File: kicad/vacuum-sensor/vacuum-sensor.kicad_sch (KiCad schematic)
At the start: 13 parts, among them J1 Conn_01x04, U1 XGZP6857A100KPGPN, U2 XGZP6857A100KPGPN, U3 MIC5233-5.0YM5-TR

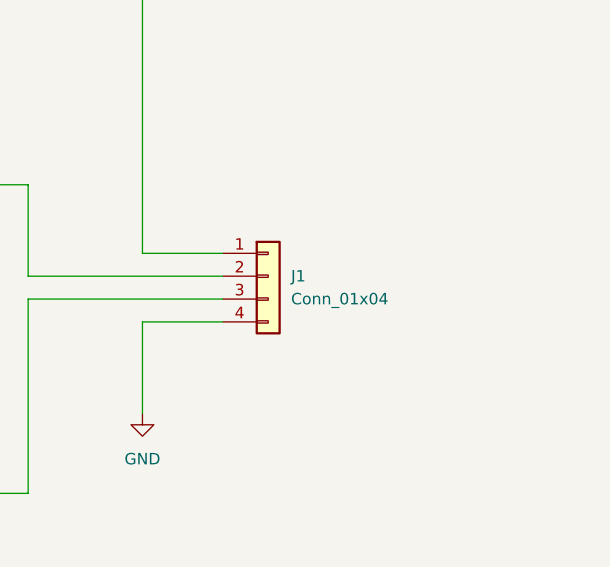
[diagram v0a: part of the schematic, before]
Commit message: Added second optionalk connector
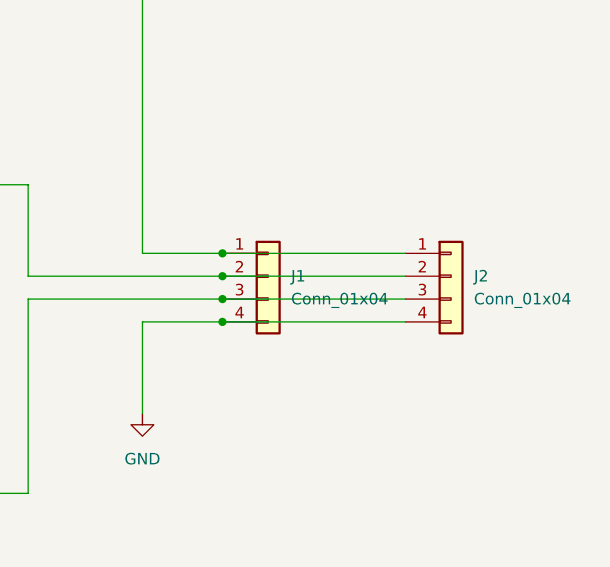
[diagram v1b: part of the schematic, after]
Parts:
- added J2: Conn_01x04, Connector_JST:JST_XH_S4B-XH-A_1x04_P2.50mm_Horizontal, symbol Connector_Generic:Conn_01x04
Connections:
- net GND: now also J2.4 (Pin_4)
- net at C6.1, J1.3 (Pin_3), R3.2: now also J2.3 (Pin_3)
- net at C5.1, J1.2 (Pin_2), R2.2: now also J2.2 (Pin_2)
- net at J1.1 (Pin_1), R1.2: now also J2.1 (Pin_1)
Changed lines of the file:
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@@
 (kicad_sch (version 20211123) (generator eeschema)
   (paper "A4")
+  (junction (at 203.2 95.25) (diameter 0) (color 0 0 0 0)
+  )
   (junction (at 115.57 43.18) (diameter 0) (color 0 0 0 0)
   )
+  (junction (at 203.2 92.71) (diameter 0) (color 0 0 0 0)
+  )
   (junction (at 91.44 97.79) (diameter 0) (color 0 0 0 0)
   )
   (junction (at 77.47 63.5) (diameter 0) (color 0 0 0 0)
   )
+  (junction (at 203.2 87.63) (diameter 0) (color 0 0 0 0)
+  )
   (junction (at 123.19 80.01) (diameter 0) (color 0 0 0 0)
   )
   (junction (at 91.44 63.5) (diameter 0) (color 0 0 0 0)
+  )
+  (junction (at 203.2 90.17) (diameter 0) (color 0 0 0 0)
   )
   (junction (at 154.94 43.18) (diameter 0) (color 0 0 0 0)
@@
     (stroke (width 0) (type default) (color 0 0 0 0))
   )
+  (wire (pts (xy 203.2 92.71) (xy 223.52 92.71))
+    (stroke (width 0) (type default) (color 0 0 0 0))
+  )
+  (wire (pts (xy 203.2 90.17) (xy 223.52 90.17))
+    (stroke (width 0) (type default) (color 0 0 0 0))
+  )
   (wire (pts (xy 181.61 80.01) (xy 123.19 80.01))
     (stroke (width 0) (type default) (color 0 0 0 0))
@@
     (stroke (width 0) (type default) (color 0 0 0 0))
   )
+  (wire (pts (xy 203.2 87.63) (xy 223.52 87.63))
+    (stroke (width 0) (type default) (color 0 0 0 0))
+  )
   (wire (pts (xy 181.61 90.17) (xy 181.61 80.01))
     (stroke (width 0) (type default) (color 0 0 0 0))
@@
   )
   (wire (pts (xy 101.6 97.79) (xy 91.44 97.79))
+    (stroke (width 0) (type default) (color 0 0 0 0))
+  )
+  (wire (pts (xy 203.2 95.25) (xy 223.52 95.25))
     (stroke (width 0) (type default) (color 0 0 0 0))
   )
@@
     (pin "5")
   )
+  (symbol (lib_id "Connector_Generic:Conn_01x04") (at 228.6 90.17 0) (unit 1)
+    (in_bom yes) (on_board yes) (fields_autoplaced)
+    (property "Reference" "J2" (id 0) (at 231.14 90.1699 0)
+      (effects (font (size 1.27 1.27)) (justify left))
+    )
+    (property "Value" "Conn_01x04" (id 1) (at 231.14 92.7099 0)
+      (effects (font (size 1.27 1.27)) (justify left))
+    )
+    (property "Footprint" "Connector_JST:JST_XH_S4B-XH-A_1x04_P2.50mm_Horizontal" (id 2) (at 228.6 90.17 0)
+      (effects (font (size 1.27 1.27)) hide)
+    )
+    (property "Datasheet" "~" (id 3) (at 228.6 90.17 0)
+      (effects (font (size 1.27 1.27)) hide)
+    )
+    (pin "1")
+    (pin "2")
+    (pin "3")
+    (pin "4")
+  )
   (symbol (lib_id "power:GND") (at 91.44 124.46 0) (unit 1)
     (in_bom yes) (on_board yes) (fields_autoplaced)
@@
       (reference "J1") (unit 1) (value "Conn_01x04") (footprint "Connector_JST:JST_XH_B4B-XH-A_1x04_P2.50mm_Vertical")
     )
+    (path "/b8382866-f10b-4adc-84fc-f6e5dd44681b"
+      (reference "J2") (unit 1) (value "Conn_01x04") (footprint "Connector_JST:JST_XH_S4B-XH-A_1x04_P2.50mm_Horizontal")
+    )
     (path "/974ce053-1a09-4ebf-b603-d7b0fff8bf5c"

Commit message: Minor changes
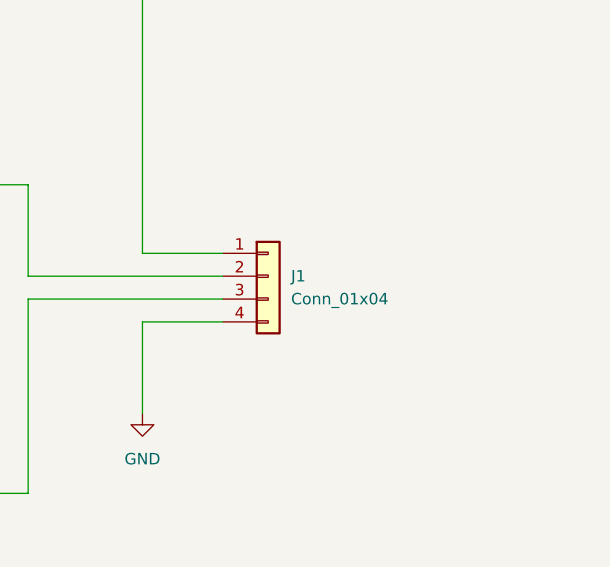
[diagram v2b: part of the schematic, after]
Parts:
- removed J2: Conn_01x04, Connector_JST:JST_XH_S4B-XH-A_1x04_P2.50mm_Horizontal, symbol Connector_Generic:Conn_01x04
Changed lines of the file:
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@@
 (kicad_sch (version 20211123) (generator eeschema)
   (paper "A4")
-  (junction (at 203.2 95.25) (diameter 0) (color 0 0 0 0)
-  )
   (junction (at 115.57 43.18) (diameter 0) (color 0 0 0 0)
   )
-  (junction (at 203.2 92.71) (diameter 0) (color 0 0 0 0)
-  )
   (junction (at 91.44 97.79) (diameter 0) (color 0 0 0 0)
   )
   (junction (at 77.47 63.5) (diameter 0) (color 0 0 0 0)
   )
-  (junction (at 203.2 87.63) (diameter 0) (color 0 0 0 0)
-  )
   (junction (at 123.19 80.01) (diameter 0) (color 0 0 0 0)
   )
   (junction (at 91.44 63.5) (diameter 0) (color 0 0 0 0)
-  )
-  (junction (at 203.2 90.17) (diameter 0) (color 0 0 0 0)
   )
   (junction (at 154.94 43.18) (diameter 0) (color 0 0 0 0)
@@
     (stroke (width 0) (type default) (color 0 0 0 0))
   )
-  (wire (pts (xy 203.2 92.71) (xy 223.52 92.71))
-    (stroke (width 0) (type default) (color 0 0 0 0))
-  )
-  (wire (pts (xy 203.2 90.17) (xy 223.52 90.17))
-    (stroke (width 0) (type default) (color 0 0 0 0))
-  )
   (wire (pts (xy 181.61 80.01) (xy 123.19 80.01))
     (stroke (width 0) (type default) (color 0 0 0 0))
@@
     (stroke (width 0) (type default) (color 0 0 0 0))
   )
-  (wire (pts (xy 203.2 87.63) (xy 223.52 87.63))
-    (stroke (width 0) (type default) (color 0 0 0 0))
-  )
   (wire (pts (xy 181.61 90.17) (xy 181.61 80.01))
     (stroke (width 0) (type default) (color 0 0 0 0))
@@
   )
   (wire (pts (xy 101.6 97.79) (xy 91.44 97.79))
-    (stroke (width 0) (type default) (color 0 0 0 0))
-  )
-  (wire (pts (xy 203.2 95.25) (xy 223.52 95.25))
     (stroke (width 0) (type default) (color 0 0 0 0))
   )
@@
     (pin "5")
   )
-  (symbol (lib_id "Connector_Generic:Conn_01x04") (at 228.6 90.17 0) (unit 1)
-    (in_bom yes) (on_board yes) (fields_autoplaced)
-    (property "Reference" "J2" (id 0) (at 231.14 90.1699 0)
-      (effects (font (size 1.27 1.27)) (justify left))
-    )
-    (property "Value" "Conn_01x04" (id 1) (at 231.14 92.7099 0)
-      (effects (font (size 1.27 1.27)) (justify left))
-    )
-    (property "Footprint" "Connector_JST:JST_XH_S4B-XH-A_1x04_P2.50mm_Horizontal" (id 2) (at 228.6 90.17 0)
-      (effects (font (size 1.27 1.27)) hide)
-    )
-    (property "Datasheet" "~" (id 3) (at 228.6 90.17 0)
-      (effects (font (size 1.27 1.27)) hide)
-    )
-    (pin "1")
-    (pin "2")
-    (pin "3")
-    (pin "4")
-  )
   (symbol (lib_id "power:GND") (at 91.44 124.46 0) (unit 1)
     (in_bom yes) (on_board yes) (fields_autoplaced)
@@
       (reference "J1") (unit 1) (value "Conn_01x04") (footprint "Connector_JST:JST_XH_B4B-XH-A_1x04_P2.50mm_Vertical")
     )
-    (path "/b8382866-f10b-4adc-84fc-f6e5dd44681b"
-      (reference "J2") (unit 1) (value "Conn_01x04") (footprint "Connector_JST:JST_XH_S4B-XH-A_1x04_P2.50mm_Horizontal")
-    )
     (path "/974ce053-1a09-4ebf-b603-d7b0fff8bf5c"
